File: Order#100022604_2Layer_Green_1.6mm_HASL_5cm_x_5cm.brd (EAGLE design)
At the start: 49.5 x 50 mm, 29 parts, among them IC1 REG1117, J1 POWER_JACKSLT, T1 BC337, X1 22-23-2031, X2 22-23-2031, X3 22-23-2031, X5 22-23-2041

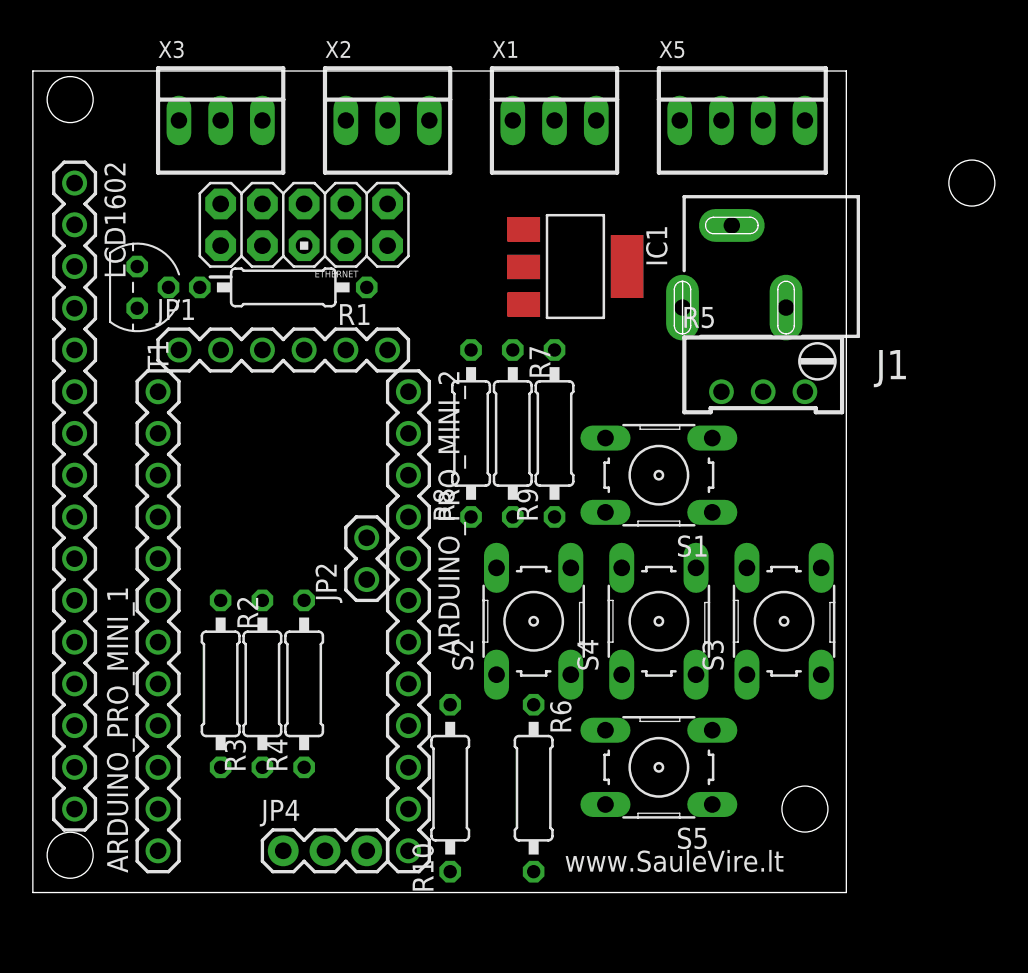
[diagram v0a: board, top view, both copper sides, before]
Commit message: Finito, paruo6ta siuntimui
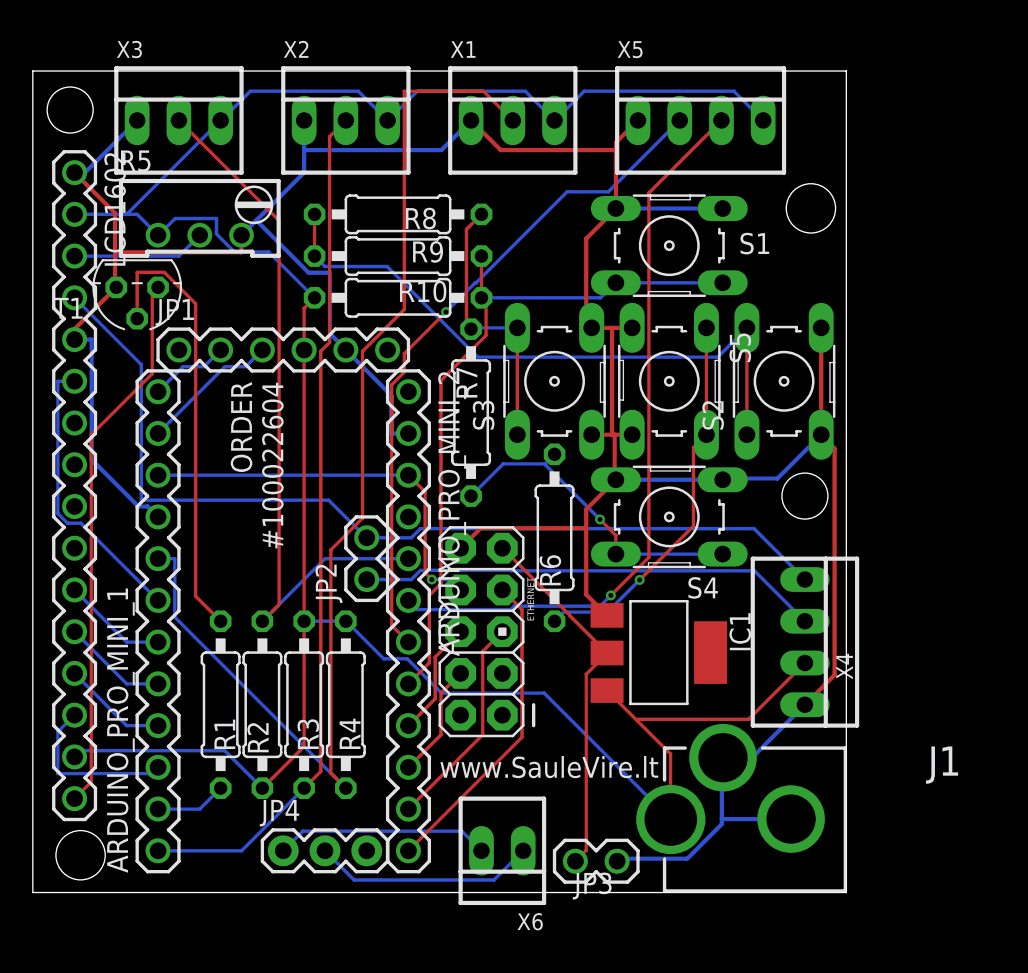
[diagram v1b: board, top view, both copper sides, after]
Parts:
- added JP3: GND 3.3V, SparkFun:1X02
- added X4: GND A5 A4 VCC, con-molex:22-23-2041
- added X6: A6 A7, con-molex:22-23-2021
- ETHERNET: value M05X2PTH -> ENC25J60
- J1: value POWER_JACKSLT -> POWER; device SparkFun-Connectors:POWER_JACK_SLOT -> SparkFun-Connectors:POWER_JACK_PTH_LOCK
- JP1: value tx rx vcc gnd -> DTR TX RX VCC GDN
- R2: value 4k7 -> 4k7
- S1: value (none) -> Right
- S2: value (none) -> Up
- S3: value (none) -> Down
- S4: value (none) -> Left
- S5: value (none) -> Select
- X1: value 22-23-2031 -> VCC D2 GND
- X2: value 22-23-2031 -> VCC D9 GND
- X3: value 22-23-2031 -> VCC A3 GND
- X5: value 22-23-2041 -> VCC A2 A1 GND
- moved R5 35.6 mm to (10.2, 41.3)
- moved R10 30.0 mm to (22.2, 36.2), turned to 180 degrees
- moved J1 28.6 mm to (52.7, 4.45)
- moved ETHERNET 27.0 mm to (27.3, 15.9), turned to 180 degrees
- moved R1 25.7 mm to (11.4, 11.4), turned to 270 degrees
- moved IC1 24.0 mm to (38.1, 14.6)
- moved S5 23.5 mm to (38.7, 31.1), turned to 270 degrees
- moved S2 21.1 mm to (45.7, 31.1)
- moved S3 20.2 mm to (31.8, 31.1)
- moved R6 15.3 mm to (31.8, 21.6)
- moved R9 14.4 mm to (22.2, 38.7), turned to 0 degrees
- moved R8 14.1 mm to (22.2, 41.3), turned to 180 degrees
- moved S1 14.0 mm to (38.7, 39.4)
- moved S4 6.38 mm to (38.7, 22.9), turned to 180 degrees
- moved R2 2.84 mm to (14.0, 11.4)
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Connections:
- new net A6: JP4.2, X6.1
- new net A7: JP4.1, X6.2
- net 3.3V: now also JP3.1
- net A3: now also R2.2, X3.2
- net A4: now also X4.2; no longer R2.2, X1.2
- net A5: now also X4.1
- net D2: now also X1.2; no longer X3.2
- net GND: now also J1.GND, J1.GNDBREAK, JP3.2, X4.4
- net VCC: now also J1.PWR, X4.3
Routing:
- net GND: track 0.00 -> 199.1 mm
- net VCC: track 0.00 -> 155.7 mm
- net D2: track 0.00 -> 71.3 mm
- net A5: track 0.00 -> 56.8 mm
- net D9: track 0.00 -> 52.2 mm
- net A2: track 0.00 -> 44.6 mm, vias 0 -> 1
- net A3: track 0.00 -> 43.9 mm
- net A0: track 0.00 -> 43.2 mm
- net A1: track 0.00 -> 40.9 mm, vias 0 -> 1
- net N$11: track 0.00 -> 38.6 mm
- net LCD16: track 0.00 -> 33.2 mm
- net A4: track 0.00 -> 28.2 mm
- net N$4: track 0.00 -> 27.1 mm
- net RESET: track 0.00 -> 24.2 mm, vias 0 -> 1
- net N$5: track 0.00 -> 23.2 mm, vias 0 -> 1
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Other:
- board text added: "ORDER #100022604"
- board text added: "www.SauleVire.lt Saules kolektoriaus valdiklis V1.2 www.SauleVire.lt/en Solar collector controller V1.2"
